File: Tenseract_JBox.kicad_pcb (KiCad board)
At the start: 2 copper layers, 62 x 24 mm, 19 parts, among them J1 MR30PW-M, J10 Conn_01x04_Pin, J11 Conn_01x04_Pin, J12 Conn_01x04_Pin, J15 TEST_IN, J16 TEST_OUT, J17 DO_SEL, J19 DO_SEL, J2 WS2815_01_IN, J3 WS2815_02_IN, J4 MR30PW-FB, J5 WS2815_01_OUT, J6 WS2815_02_OUT, J8 Conn_01x04_Pin

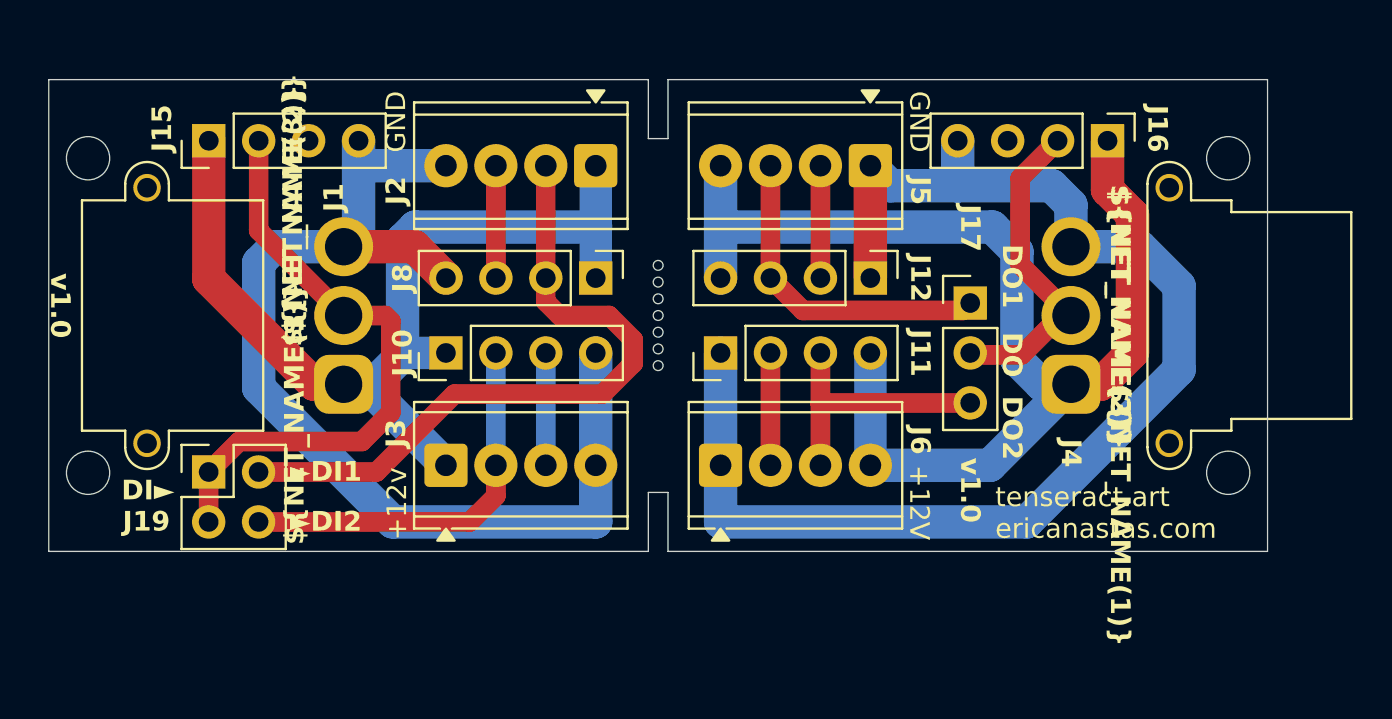
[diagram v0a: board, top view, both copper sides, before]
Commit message: Finished 2nd pcb
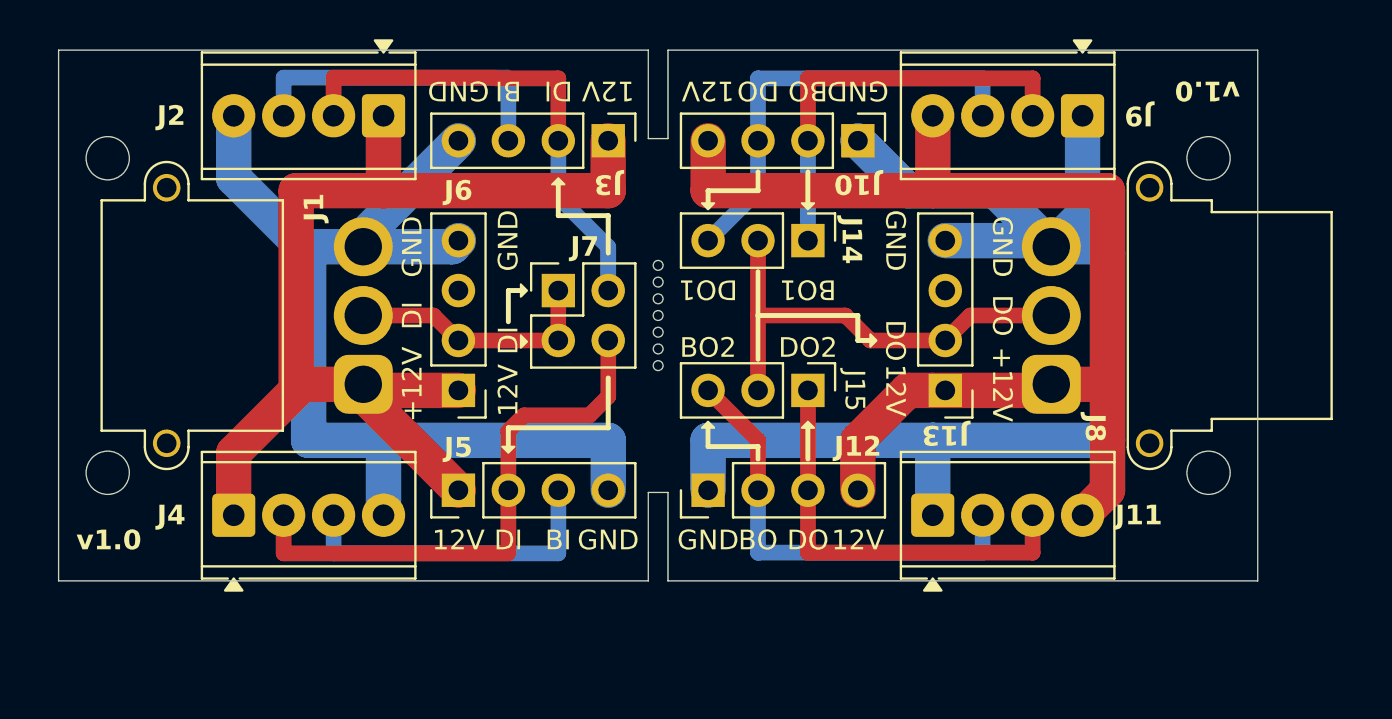
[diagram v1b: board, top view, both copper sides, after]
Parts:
- added J15: DO_SEL2, Connector_PinHeader_2.54mm:PinHeader_1x03_P2.54mm_Vertical, F.Cu at (118.6, 53.8)
- J14: renamed from J17; value DO_SEL -> DO_SEL1
- moved J7 20.0 mm to (105.9, 48.7)
- moved J6 18.0 mm to (100.8, 53.8), turned to 180 degrees
- moved J13 15.1 mm to (125.6, 53.8), turned to 180 degrees
- moved J11 11.1 mm to (125.0, 60.2)
- moved J2 11.1 mm to (97.0, 39.8)
- moved J4 11.1 mm to (89.4, 60.2)
- moved J9 11.1 mm to (132.6, 39.8)
- moved J14 8.84 mm to (118.6, 46.2), turned to -90 degrees
- moved J10 7.01 mm to (121.2, 41.1)
- moved J5 7.01 mm to (100.8, 58.9)
- moved J12 7.01 mm to (113.5, 58.9)
- moved J3 7.01 mm to (108.5, 41.1)
- moved J1 1.00 mm to (96.0, 53.5)
- moved J8 1.00 mm to (131.0, 53.5)
- moved REF** 1.00 mm to (139.0, 58.0)
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- renumbered J12 to J10, J6 to J11, J11 to J12, J16 to J13, J8 to J3, J3 to J4, J10 to J5, J15 to J6, J19 to J7, J4 to J8, J5 to J9
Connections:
- net BI1 renamed /BI1
- net BO2 renamed /BO2
- net DI renamed /DI
- net DI2 renamed /DI2
- net DO renamed /DO
- J10 pad 2: B01 -> /BO1
- J10 pad 3: DO1 -> /DO1
- J11 pad 3: DO2 -> /DO2
- J12 pad 3: DO2 -> /DO2
- J14 pad 1: DO1 -> /BO1
- J14 pad 3: DO2 -> /DO1
- J9 pad 2: B01 -> /BO1
- J9 pad 3: DO1 -> /DO1
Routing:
- net /DO1: track 0.00 -> 22.6 mm
- net /DO2: track 0.00 -> 21.6 mm
- net /BO1: track 0.00 -> 21.6 mm
- net /DI: track 30.9 -> 13.0 mm
- net /BO2: track 5.71 -> 22.6 mm
- net DO1: track 16.7 -> 0.00 mm
- net DO2: track 13.4 -> 0.00 mm
- net /BI2: track 5.71 -> 16.6 mm
- net /BI1: track 5.71 -> 16.6 mm
- net /DI1: track 34.7 -> 25.2 mm
- net /DI2: track 19.9 -> 28.6 mm
- net /DO: track 16.7 -> 23.6 mm
- net B01: track 5.71 -> 0.00 mm
- net GND: track 122.5 -> 119.6 mm
- net +12V: track 113.4 -> 115.1 mm
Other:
- board size 62 x 24 mm -> 61 x 27 mm
- board text added: "12V"
- board text added: "BI"
- board text added: "BO"
- board text added: "BO1"
- board text added: "BO2"
- board text added: "DI"
- board text added: "ericanastas.com"
- board text added: "tenseract.art"
- board text removed: "+12v"
- board text removed: "DI►"
- board text removed: "tenseract.art ericanastas.com"
- board text removed: "►DI1"
- board text removed: "►DI2"
